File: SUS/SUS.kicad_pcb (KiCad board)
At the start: 4 copper layers, 117.7 x 30.4 mm, 72 parts, among them J1 ESP32_Connector_0, J2 ESP32_Connector_1, J3 I2C, J4 I2C, J5 I2C, J6 ADC, J7 WS, U1 TJA1051T, U2 ADS8320EB_250, U3 ICM-42688-P, U4 S1001-46R, U5 S1001-46R, U6 S1001-46R

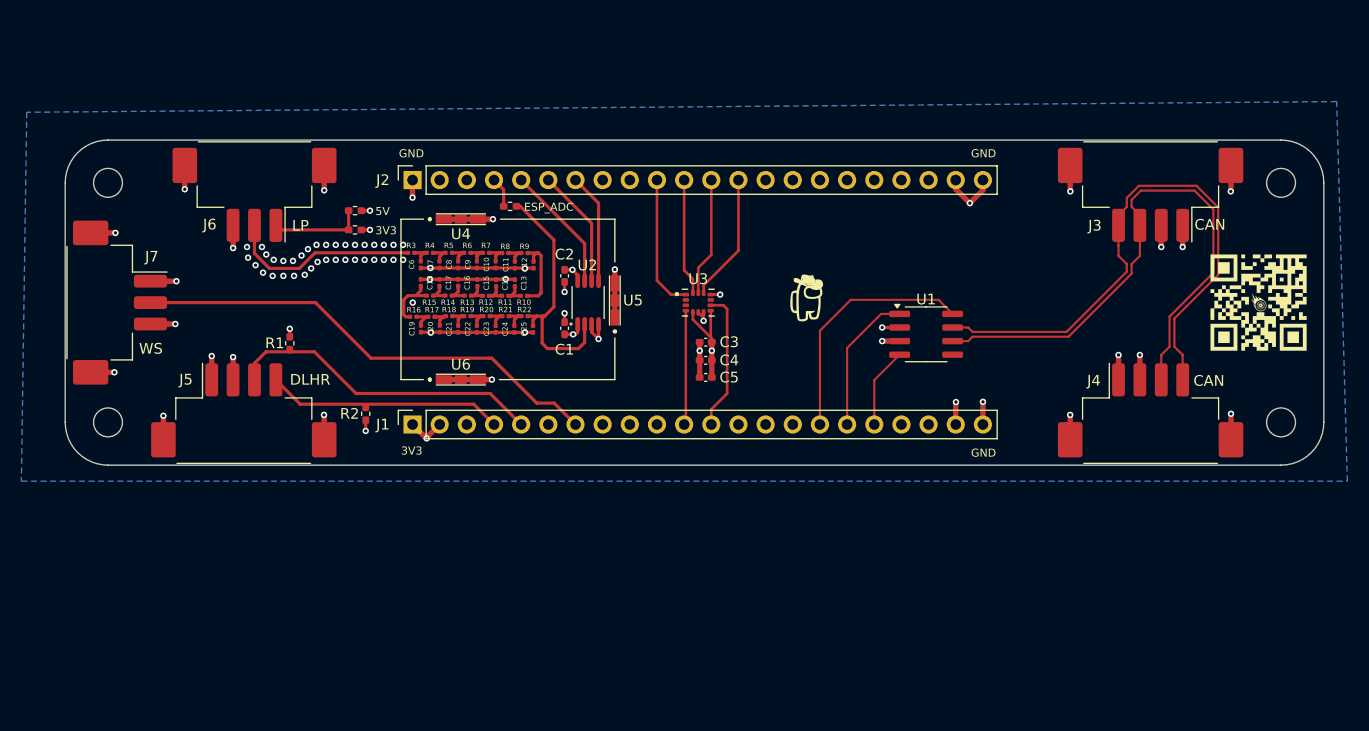
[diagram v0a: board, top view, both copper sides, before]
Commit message: Complete re-design. Readme still needs to be updated.
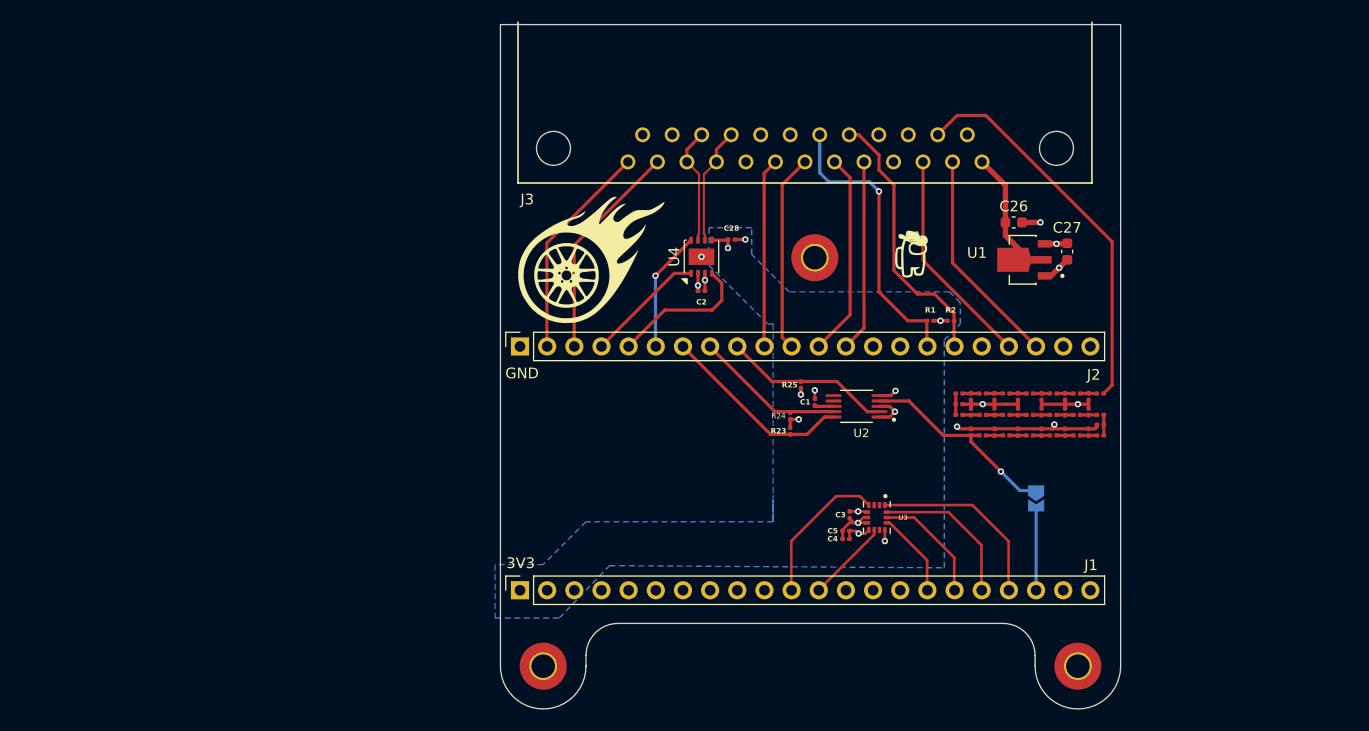
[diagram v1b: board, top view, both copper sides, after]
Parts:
- removed the G*** at (106.8, 58.1)
- removed the G*** at (106.6, 59.9)
- removed the G*** at (148.9, 60.0)
- removed the G*** at (96.6, 60.1)
- removed H4: MountingHole, MountingHole:MountingHole_2.7mm_M2.5
- removed J4, J5: I2C, Connector_Hirose:Hirose_DF3EA-04P-2H_1x04-1MP_P2.00mm_Horizontal
- removed J6: ADC, Connector_Hirose:Hirose_DF3EA-03P-2H_1x03-1MP_P2.00mm_Horizontal
- removed J7: WS, Connector_Hirose:Hirose_DF3EA-03P-2H_1x03-1MP_P2.00mm_Horizontal
- removed R27: 0, Resistor_SMD:R_0402_1005Metric_Pad0.72x0.64mm_HandSolder
- removed U5, U6: S1001-46R, S1001-46R:S100146R
- added C26: 10μF, Capacitor_SMD:C_0603_1608Metric, F.Cu at (126.0, 52.5)
- added C27: 10μF, Capacitor_SMD:C_0603_1608Metric, F.Cu at (131.0, 55.2)
- added C28: 0.1μF, Capacitor_SMD:C_0201_0603Metric, F.Cu at (99.6, 54.1)
- added G***: LOGO, LOGO, F.Cu at (116.4, 55.8)
- added G***: LOGO, LOGO, F.Cu at (86.5, 56.0)
- added G***: LOGO, LOGO, F.Cu at (116.6, 54.0)
- added JP1: SolderJumper_2_Open, Jumper:SolderJumper-2_P1.3mm_Open_TrianglePad1.0x1.5mm, B.Cu at (128.1, 78.3)
- added R25: 10k, Capacitor_SMD:C_0201_0603Metric, F.Cu at (106.1, 67.7)
- C1: value 10μF -> 0.1μF; footprint Capacitor_SMD:C_0402_1005Metric_Pad0.74x0.62mm_HandSolder -> Capacitor_SMD:C_0201_0603Metric
- C2: value 1μF -> 0.1μF; footprint Capacitor_SMD:C_0402_1005Metric_Pad0.74x0.62mm_HandSolder -> Capacitor_SMD:C_0201_0603Metric
- C3: value 2.2μF -> 10nF; footprint Capacitor_SMD:C_0402_1005Metric_Pad0.74x0.62mm_HandSolder -> Capacitor_SMD:C_0201_0603Metric
- C4: value 0.1μF -> 2.2μF; footprint Capacitor_SMD:C_0402_1005Metric_Pad0.74x0.62mm_HandSolder -> Capacitor_SMD:C_0201_0603Metric
- C5: footprint Capacitor_SMD:C_0402_1005Metric_Pad0.74x0.62mm_HandSolder -> Capacitor_SMD:C_0201_0603Metric
- H1, H2, H3: value MountingHole -> MountingHole_Pad; footprint MountingHole:MountingHole_2.7mm_M2.5 -> MountingHole:MountingHole_2.2mm_M2_Pad_TopOnly
- J3: value I2C -> D25P13A4GV00LF; footprint Connector_Hirose:Hirose_DF3EA-04P-2H_1x04-1MP_P2.00mm_Horizontal -> D25:CONN_D25P_AMP
- R1, R2: footprint Resistor_SMD:R_0402_1005Metric_Pad0.72x0.64mm_HandSolder -> Capacitor_SMD:C_0201_0603Metric
- R23, R24: value 0 -> 10k; footprint Resistor_SMD:R_0402_1005Metric_Pad0.72x0.64mm_HandSolder -> Capacitor_SMD:C_0201_0603Metric
- U1: value TJA1051T -> HT7333; footprint Package_SO:SOIC-8_3.9x4.9mm_P1.27mm -> HT7333:IC_HT7333
- U2: value ADS8320EB_250 -> ADS1015IDGSR; footprint ADS8320EB_250:DGK0008A_L -> ADC:SOP50P490X110-10N
- U3: footprint IMU:ICM-42688-P -> IMU:PQFN50P300X250X97-14N
- U4: value S1001-46R -> TJA1051TK-3; footprint S1001-46R:S100146R -> Package_DFN_QFN:DFN-8-1EP_3x3mm_P0.65mm_EP1.55x2.4mm
- moved H3 101.3 mm to (132.0, 94.0)
- moved R3 65.8 mm to (134.1, 68.5), turned to 0 degrees
- moved R16 64.9 mm to (134.1, 70.5)
- moved C19 64.2 mm to (134.1, 71.4), turned to 0 degrees
- moved C6 63.7 mm to (133.0, 68.8)
- moved C18 63.6 mm to (133.0, 70.2)
- moved R17 63.5 mm to (134.1, 72.4), turned to 0 degrees
- moved R4 61.9 mm to (131.9, 68.5), turned to 0 degrees
- moved R15 61.5 mm to (131.9, 70.5), turned to 180 degrees
- moved C20 61.4 mm to (133.0, 72.1), turned to -90 degrees
- moved R1 59.9 mm to (118.2, 61.7), turned to 180 degrees
- moved C7 59.8 mm to (130.8, 68.8)
- moved R18 59.8 mm to (131.9, 72.4), turned to 0 degrees
- moved C17 59.7 mm to (130.8, 70.2)
- moved R5 58.0 mm to (129.7, 68.5), turned to 0 degrees
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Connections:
- C1 pad 1: +5V -> 5V
- C2 pad 1: +3.3V -> +5V
- J1 pad 16: CAN_S -> IMU_CS
- J1 pad 17: CAN_TX -> IMU_SCL
- J1 pad 18: CAN_RX -> IMU_MOSI
- J1 pad 19: unconnected-(J1-Pin_19-Pad19) -> IMU_MISO
- J1 pad 20: unconnected-(J1-Pin_20-Pad20) -> ESP_ADC
- J1 pad 4: I2C_SDA -> unconnected-(J1-Pin_4-Pad4)
- J1 pad 5: I2C_SCL -> unconnected-(J1-Pin_5-Pad5)
- J1 pad 7: /WS_IN -> unconnected-(J1-Pin_7-Pad7)
- J2 pad 10: IMU_MISO -> GPIO 38
- J2 pad 11: IMU_MOSI -> GPIO 37
- J2 pad 12: IMU_SCK -> GPIO 36
- J2 pad 13: IMU_CS -> GPIO 35
- J2 pad 16: unconnected-(J2-Pin_16-Pad16) -> I2C_SCL
- J2 pad 17: unconnected-(J2-Pin_17-Pad17) -> I2C_SDA
- J2 pad 19: unconnected-(J2-Pin_19-Pad19) -> GPIO 20
- J2 pad 2: unconnected-(J2-Pin_2-Pad2) -> TX
- J2 pad 20: unconnected-(J2-Pin_20-Pad20) -> GPIO 19
- J2 pad 3: unconnected-(J2-Pin_3-Pad3) -> RX
- J2 pad 4: Net-(J2-Pin_4) -> CAN_TX
- J2 pad 5: A_SCK -> CAN_RX
- J2 pad 6: A_MISO -> CAN_S
- J2 pad 7: A_CS -> A_SCL
- J2 pad 8: unconnected-(J2-Pin_8-Pad8) -> A_SDA
- J2 pad 9: unconnected-(J2-Pin_9-Pad9) -> A_CS
- J3 pad 1: +5V -> +12V
- J3 pad 2: GND -> GPIO 19
- J3 pad 3: CAN- -> GPIO 20
- J3 pad 4: CAN+ -> GND
- R23 pad 2: Net-(J6-Pin_1) -> A_SCL
- R24 pad 1: +5V -> +3.3V
- R24 pad 2: Net-(J6-Pin_1) -> A_SDA
- U1 pad 1: CAN_TX -> GND
- U1 pad 2: GND -> +12V
- U2 pad 1: +5V -> GND
- U2 pad 2: AA_out -> A_CS
- U2 pad 4: GND -> AA_out
- U2 pad 5: A_CS -> GND
- U2 pad 6: A_MISO -> unconnected-(U2-AIN2-Pad6)
- U2 pad 7: A_SCK -> unconnected-(U2-AIN3-Pad7)
- U2 pad 8: +3.3V -> 5V
- U3 pad 13: IMU_SCK -> IMU_SCL
- U4 pad 1: GND -> CAN_TX
- U4 pad 3: GND -> +5V
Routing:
- net GND: track 99.6 -> 47.6 mm, vias 71 -> 14
- net /WS_IN: track 44.5 -> 0.00 mm
- net CAN+: track 53.4 -> 10.9 mm
- net CAN-: track 52.6 -> 11.0 mm
- net GPIO 20: track 0.00 -> 20.6 mm
- net GPIO 19: track 0.00 -> 20.5 mm
- net RX: track 0.00 -> 20.5 mm
- net TX: track 0.00 -> 20.4 mm
- net GPIO 36: track 0.00 -> 19.1 mm
- net GPIO 37: track 0.00 -> 18.5 mm
- net A_In: track 18.1 -> 36.5 mm
- net A_SCL: track 0.00 -> 18.2 mm
- net GPIO 35: track 0.00 -> 18.0 mm
- net GPIO 38: track 0.00 -> 17.7 mm
- net A_SDA: track 0.00 -> 14.1 mm
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- added copper zone on B.Cu, net +3.3V
- added copper zone on In1.Cu, net +5V
- removed copper zone on In1.Cu, net +3.3V
- removed copper zone on B.Cu, net +5V
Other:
- board size 117.7 x 30.4 mm -> 58 x 64 mm
- board text added: "12V"
- board text added: "19"
- board text added: "20"
- board text added: "35"
- board text added: "36"
- board text added: "37"
- board text added: "38"
- board text added: "A_IN"
- board text added: "CH"
- board text added: "CL"
- board text added: "NC"
- board text added: "RX"
- board text added: "SCL"
- board text added: "SDA"
- board text added: "TX"
- board text removed: "CAN"
- board text removed: "DLHR"
- board text removed: "ESP_ADC"
- board text removed: "LP"
- board text removed: "U3"
- board text removed: "WS"
